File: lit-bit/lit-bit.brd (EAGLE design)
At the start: 71 parts, among them J2 USB_MICRO_B_SMD_FEMALE, J3 ISP, U2 32U4, U3 73831, U4 ADXL345, U5 S-1335, U6 MCP7940N, U7 24FC1025, Y1 8MHz, Y2 32.768kHz, Y3 32.768kHz, Y4 16MHz

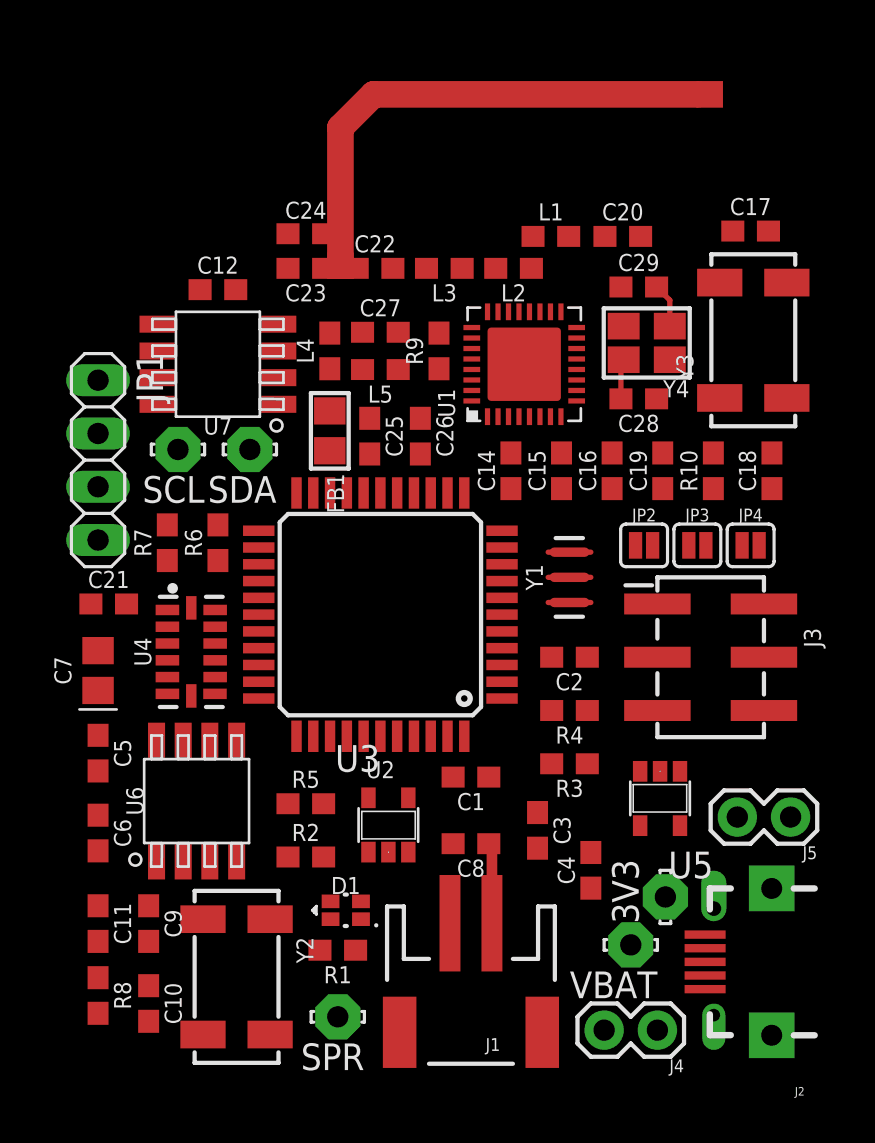
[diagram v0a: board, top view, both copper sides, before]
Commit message: acktually done with layout now, got board dimensions
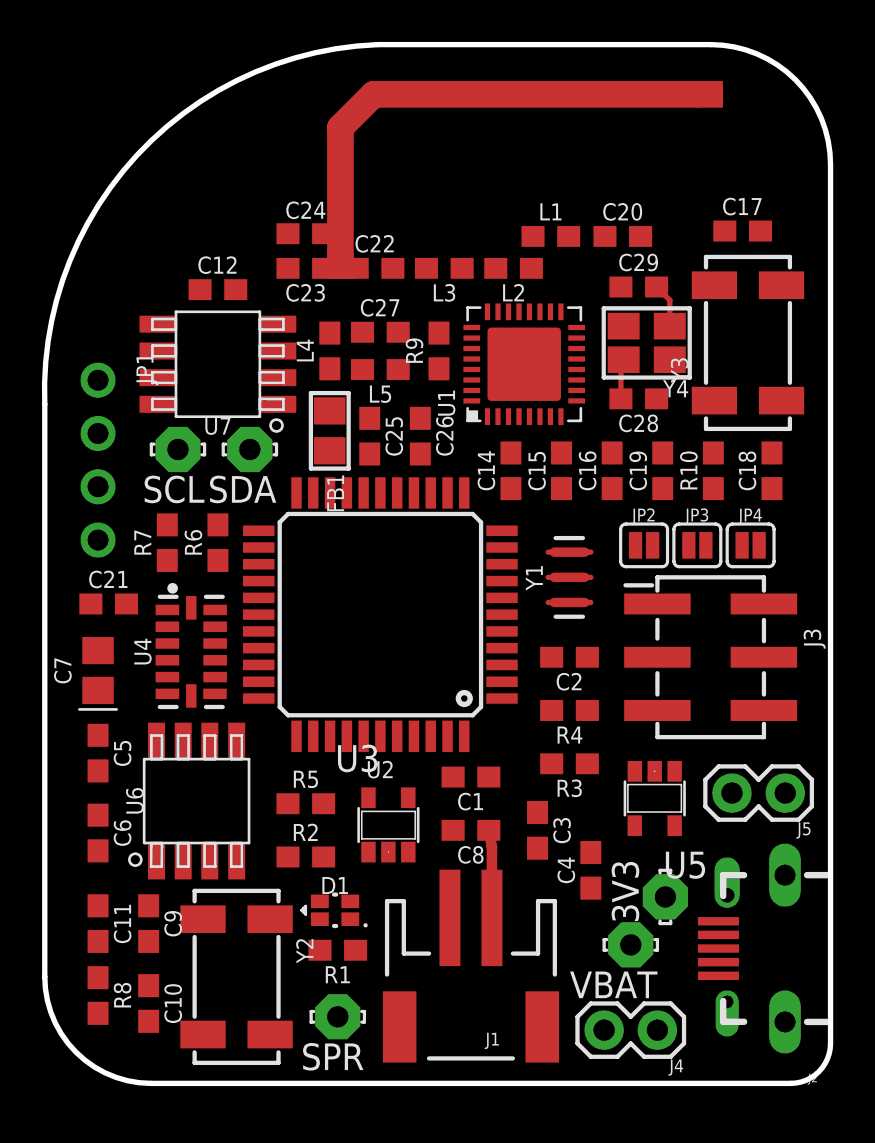
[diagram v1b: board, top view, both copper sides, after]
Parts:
- JP1: device pinhead:1X04 -> microbuilder:1X04_ROUND
- moved J5 1.17 mm to (34.7, 13.8)
- moved J2 0.90 mm to (36.8, 10.2)
- moved C8 0.63 mm to (19.7, 12.1)
- moved D1 0.51 mm to (13.2, 8.26)
- moved C17 0.38 mm to (32.6, 40.6)
- moved Y3 0.28 mm to (32.9, 35.3)
- moved U5 0.25 mm to (28.4, 13.6)
- moved J1 0.25 mm to (19.7, 4.19)
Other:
- board outline added: 37.5 x 49.5 mm
